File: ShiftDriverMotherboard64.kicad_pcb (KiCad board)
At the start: 2 copper layers, 9 parts, among them U1 ShiftDriver, U2 ShiftDriver, U3 ShiftDriver, U4 ShiftDriver, U5 ShiftDriver, U6 ShiftDriver, U7 ShiftDriver, U8 ShiftDriver, U9 TEENSY_3.6_MINIMAL

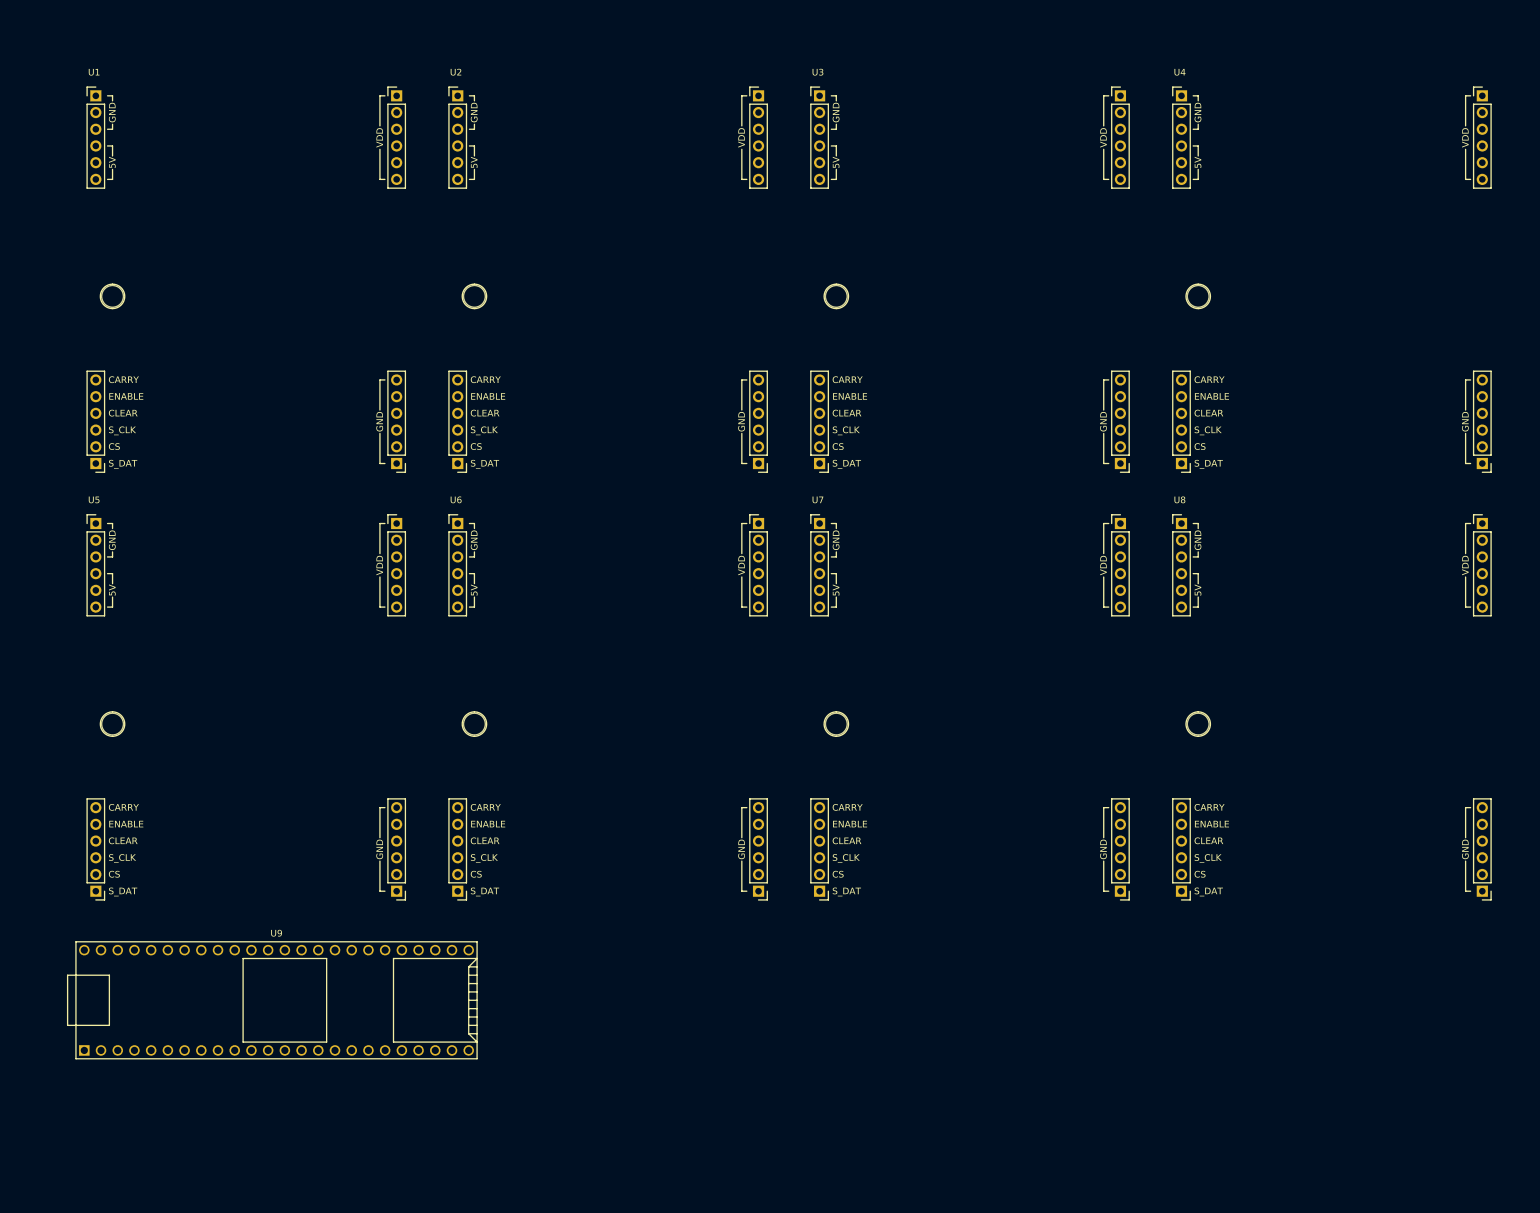
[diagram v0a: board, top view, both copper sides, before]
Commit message: first crack at layout, gonna try laying traces soon
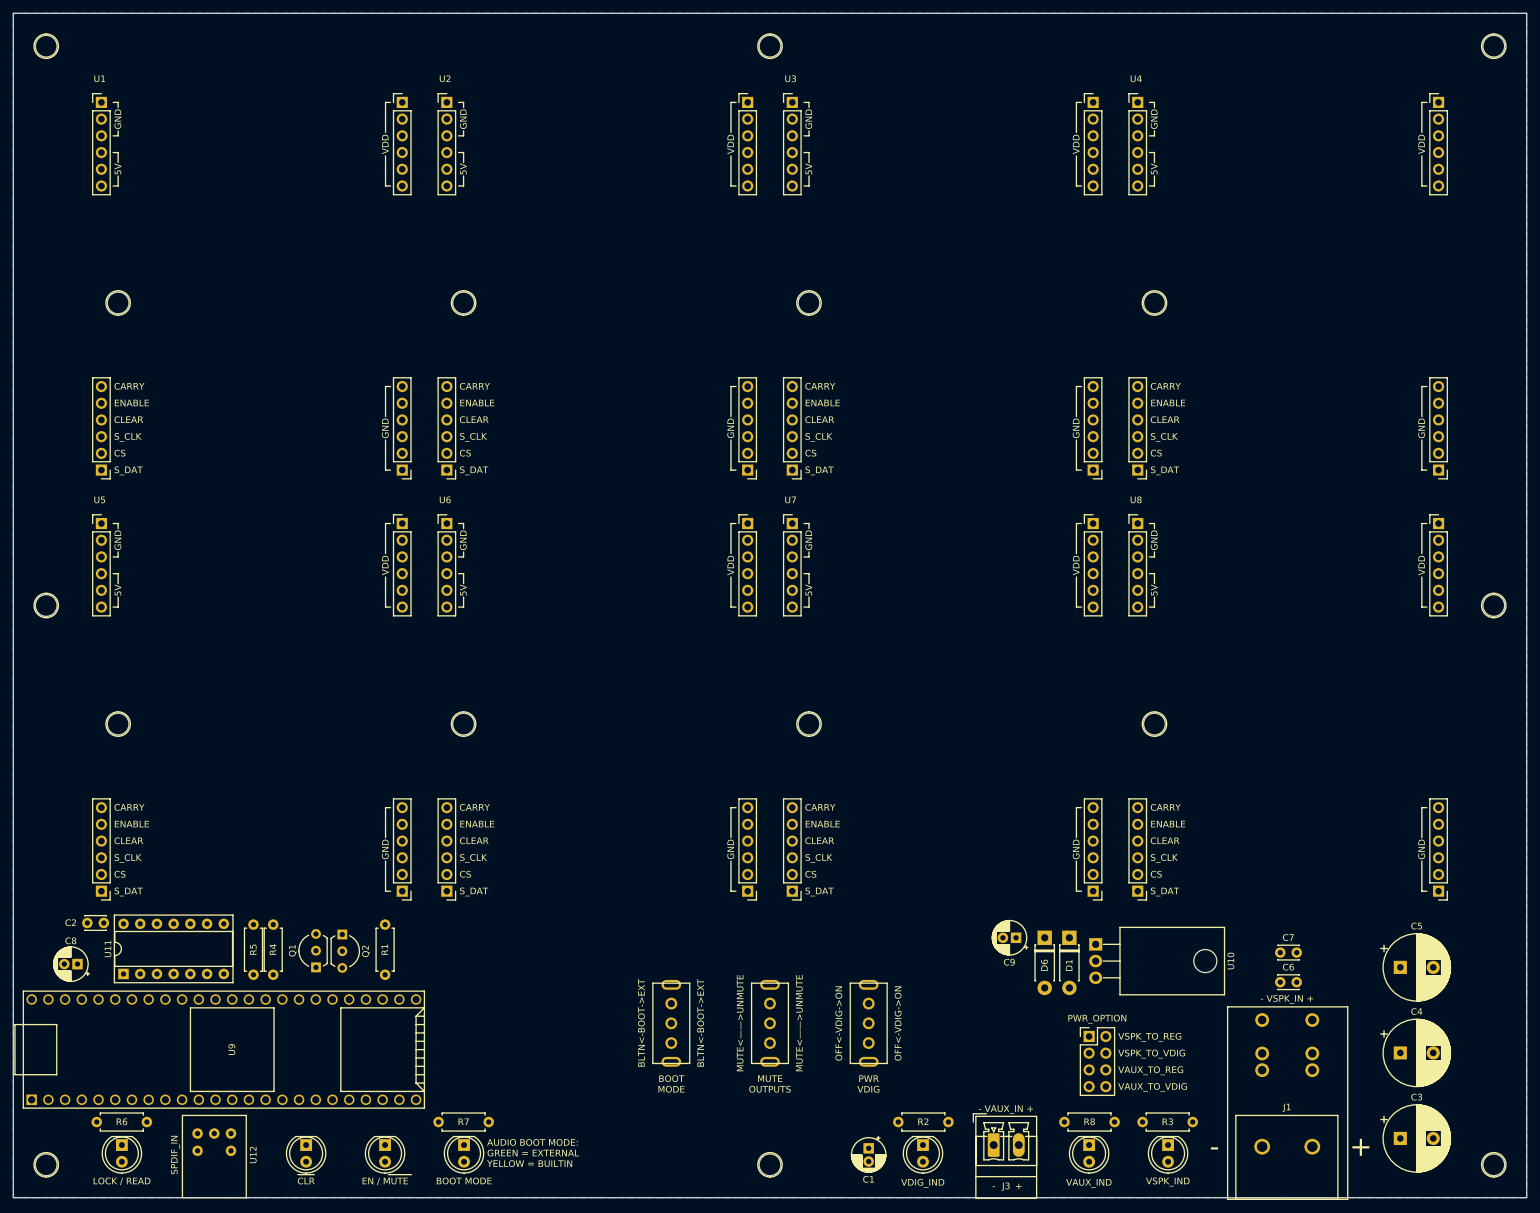
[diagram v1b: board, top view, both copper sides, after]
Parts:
- added C1: 10uf, Capacitor_THT:CP_Radial_D5.0mm_P2.00mm, F.Cu at (140.0, 182.5)
- added C2: 0.1uf, Capacitor_THT:C_Disc_D3.0mm_W2.0mm_P2.50mm, F.Cu at (21.2, 148.2)
- added C3: 470uf, Capacitor_THT:CP_Radial_D10.0mm_P5.00mm, F.Cu at (220.8, 181.0)
- added C4: 470uf, Capacitor_THT:CP_Radial_D10.0mm_P5.00mm, F.Cu at (220.8, 168.0)
- added C5: 470uf, Capacitor_THT:CP_Radial_D10.0mm_P5.00mm, F.Cu at (220.8, 155.0)
- added C6: 0.1uf, Capacitor_THT:C_Disc_D3.0mm_W2.0mm_P2.50mm, F.Cu at (202.6, 157.2)
- added C7: 0.1uf, Capacitor_THT:C_Disc_D3.0mm_W2.0mm_P2.50mm, F.Cu at (202.6, 152.8)
- added C8: 10uf, Capacitor_THT:CP_Radial_D5.0mm_P2.00mm, F.Cu at (19.8, 154.5)
- added C9: 10uf, Capacitor_THT:CP_Radial_D5.0mm_P2.00mm, F.Cu at (162.4, 150.5)
- added D1: 1N4001, Diode_THT:D_DO-41_SOD81_P7.62mm_Horizontal, F.Cu at (170.5, 150.5)
- added D2: TEENSY_PWR_IND, LED_THT:LED_D5.0mm, F.Cu at (148.2, 182.0)
- added D3: VDD_IND, LED_THT:LED_D5.0mm, F.Cu at (185.5, 182.0)
- added D4: CLR_LED, LED_THT:LED_D5.0mm, F.Cu at (54.5, 182.0)
- added D5: EN_LED, LED_THT:LED_D5.0mm, F.Cu at (66.5, 182.0)
- added D6: 1N4001, Diode_THT:D_DO-41_SOD81_P7.62mm_Horizontal, F.Cu at (166.8, 150.5)
- added D7: LOCK_IND, LED_THT:LED_D5.0mm, F.Cu at (26.5, 182.0)
- added D8: BOOT_IND, LED_THT:LED_D5.0mm, F.Cu at (78.5, 182.0)
- added D9: VDIG, LED_THT:LED_D5.0mm, F.Cu at (173.5, 182.0)
- added H3: M3/#4-40, HammerheadAudio:M3_MOUNT, F.Cu at (15.0, 185.0)
- added H3: M3/#4-40, HammerheadAudio:M3_MOUNT, F.Cu at (235.0, 100.0)
- added H3: M3/#4-40, HammerheadAudio:M3_MOUNT, F.Cu at (235.0, 185.0)
- added H3: M3/#4-40, HammerheadAudio:M3_MOUNT, F.Cu at (15.0, 100.0)
- added H3: M3/#4-40, HammerheadAudio:M3_MOUNT, F.Cu at (125.0, 15.0)
- added H3: M3/#4-40, HammerheadAudio:M3_MOUNT, F.Cu at (125.0, 185.0)
- added H3: M3/#4-40, HammerheadAudio:M3_MOUNT, F.Cu at (235.0, 15.0)
- added H3: M3/#4-40, HammerheadAudio:M3_MOUNT, F.Cu at (15.0, 15.0)
- added J1: - VSPK_IN +, HammerheadAudio:ScrewTerm+Phoenix_30A_7.62mm_1x2, F.Cu at (199.8, 163.0)
- added J2: PWR OPTION HEADER, Connector_PinHeader_2.54mm:PinHeader_2x04_P2.54mm_Vertical, F.Cu at (173.5, 165.5)
- added J3: V_TNSY_IN, HammerheadAudio:Phoenix_Stacked, F.Cu at (159.0, 182.0)
- added Q1: Q_NPN_EBC, Package_TO_SOT_THT:TO-92L_Inline_Wide, F.Cu at (56.0, 155.0)
- added Q2: Q_NPN_EBC, Package_TO_SOT_THT:TO-92L_Inline_Wide, F.Cu at (60.0, 150.0)
- added R1: 1k, HammerheadAudio:R_THT_P7.62, F.Cu at (66.5, 148.5)
- added R2: 220, HammerheadAudio:R_THT_P7.62, F.Cu at (144.5, 178.5)
- added R3: 220, HammerheadAudio:R_THT_P7.62, F.Cu at (189.2, 178.5)
- added R4: 1k, HammerheadAudio:R_THT_P7.62, F.Cu at (49.5, 148.5)
- added R5: 10k, HammerheadAudio:R_THT_P7.62, F.Cu at (46.5, 148.5)
- added R6: 1k, HammerheadAudio:R_THT_P7.62, F.Cu at (30.3, 178.5)
- added R7: 1k, HammerheadAudio:R_THT_P7.62, F.Cu at (82.2, 178.5)
- added R8: 220, HammerheadAudio:R_THT_P7.62, F.Cu at (169.8, 178.5)
- added SW1: TEENSY_PWR, HammerheadAudio:Tayda_Slide_SPDT, F.Cu at (140.0, 163.5)
- added SW2: BOOT_MODE, HammerheadAudio:Tayda_Slide_SPDT, F.Cu at (110.0, 163.5)
- added SW3: MUTE_SW, HammerheadAudio:Tayda_Slide_SPDT, F.Cu at (125.0, 163.5)
- added U10: LM7805_TO220, Package_TO_SOT_THT:TO-220-3_Horizontal_TabDown, F.Cu at (174.5, 151.5)
- added U11: CD74HC243, Package_DIP:DIP-14_W7.62mm_Socket, F.Cu at (26.8, 156.0)
- added U12: EAPLRAA4, HammerheadAudio:EAPLRAA4, F.Cu at (38.0, 180.2)
- moved U9 11.0 mm to (42.0, 167.5)
- moved U4 6.72 mm to (178.3, 21.0)
- moved U8 6.65 mm to (178.3, 85.0)
- moved U3 4.27 mm to (125.8, 21.0)
- moved U7 4.15 mm to (125.8, 85.0)
- moved U2 1.93 mm to (73.3, 21.0)
- moved U6 1.65 mm to (73.3, 85.0)
- moved U1 1.31 mm to (20.9, 21.0)
- moved U5 0.85 mm to (20.9, 85.0)
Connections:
- U1 pad 1: Net-(U1-Pad1) -> VDD
- U1 pad 2: Net-(U1-Pad2) -> +5V
- U1 pad 3: Net-(U1-Pad3) -> GND
- U1 pad 4: Net-(U1-Pad4) -> D1
- U1 pad 5: Net-(U1-Pad5) -> CS
- U1 pad 6: Net-(U1-Pad6) -> S_CLK
- U1 pad 7: Net-(U1-Pad7) -> CLR
- U1 pad 8: Net-(U1-Pad8) -> EN
- U1 pad 9: Net-(U1-Pad9) -> D2
- U2 pad 1: Net-(U2-Pad1) -> VDD
- U2 pad 2: Net-(U2-Pad2) -> +5V
- U2 pad 3: Net-(U2-Pad3) -> GND
- U2 pad 4: Net-(U2-Pad4) -> D2
- U2 pad 5: Net-(U2-Pad5) -> CS
- U2 pad 6: Net-(U2-Pad6) -> S_CLK
- U2 pad 7: Net-(U2-Pad7) -> CLR
- U2 pad 8: Net-(U2-Pad8) -> EN
- U2 pad 9: Net-(U2-Pad9) -> D3
- U3 pad 1: Net-(U3-Pad1) -> VDD
- U3 pad 2: Net-(U3-Pad2) -> +5V
- U3 pad 3: Net-(U3-Pad3) -> GND
- U3 pad 4: Net-(U3-Pad4) -> D3
- U3 pad 5: Net-(U3-Pad5) -> CS
- U3 pad 6: Net-(U3-Pad6) -> S_CLK
- U3 pad 7: Net-(U3-Pad7) -> CLR
- U3 pad 8: Net-(U3-Pad8) -> EN
- U3 pad 9: Net-(U3-Pad9) -> D4
- U4 pad 1: Net-(U4-Pad1) -> VDD
- U4 pad 2: Net-(U4-Pad2) -> +5V
- U4 pad 3: Net-(U4-Pad3) -> GND
- U4 pad 4: Net-(U4-Pad4) -> D4
- U4 pad 5: Net-(U4-Pad5) -> CS
- U4 pad 6: Net-(U4-Pad6) -> S_CLK
- U4 pad 7: Net-(U4-Pad7) -> CLR
- U4 pad 8: Net-(U4-Pad8) -> EN
- U4 pad 9: Net-(U4-Pad9) -> D5
- U5 pad 1: Net-(U5-Pad1) -> VDD
- U5 pad 2: Net-(U5-Pad2) -> +5V
- U5 pad 3: Net-(U5-Pad3) -> GND
- U5 pad 4: Net-(U5-Pad4) -> D5
- U5 pad 5: Net-(U5-Pad5) -> CS
- U5 pad 6: Net-(U5-Pad6) -> S_CLK
- U5 pad 7: Net-(U5-Pad7) -> CLR
- U5 pad 8: Net-(U5-Pad8) -> EN
- U5 pad 9: Net-(U5-Pad9) -> D6
- U6 pad 1: Net-(U6-Pad1) -> VDD
- U6 pad 2: Net-(U6-Pad2) -> +5V
- U6 pad 3: Net-(U6-Pad3) -> GND
- U6 pad 4: Net-(U6-Pad4) -> D6
- U6 pad 5: Net-(U6-Pad5) -> CS
- U6 pad 6: Net-(U6-Pad6) -> S_CLK
- U6 pad 7: Net-(U6-Pad7) -> CLR
- U6 pad 8: Net-(U6-Pad8) -> EN
- U6 pad 9: Net-(U6-Pad9) -> D7
- U7 pad 1: Net-(U7-Pad1) -> VDD
- U7 pad 2: Net-(U7-Pad2) -> +5V
- U7 pad 3: Net-(U7-Pad3) -> GND
- U7 pad 4: Net-(U7-Pad4) -> D7
- U7 pad 5: Net-(U7-Pad5) -> CS
- U7 pad 6: Net-(U7-Pad6) -> S_CLK
- U7 pad 7: Net-(U7-Pad7) -> CLR
- U7 pad 8: Net-(U7-Pad8) -> EN
- U7 pad 9: Net-(U7-Pad9) -> D8
- U8 pad 1: Net-(U8-Pad1) -> VDD
- U8 pad 2: Net-(U8-Pad2) -> +5V
- U8 pad 3: Net-(U8-Pad3) -> GND
- U8 pad 4: Net-(U8-Pad4) -> D8
- U8 pad 5: Net-(U8-Pad5) -> CS
- U8 pad 6: Net-(U8-Pad6) -> S_CLK
- U8 pad 7: Net-(U8-Pad7) -> CLR
- U8 pad 8: Net-(U8-Pad8) -> EN
- U9 pad 1: Net-(U9-Pad1) -> GND
- U9 pad 11: Net-(U9-Pad11) -> CLR_PIN
- U9 pad 12: Net-(U9-Pad12) -> CS_PIN
- U9 pad 13: Net-(U9-Pad13) -> DAT_PIN
- U9 pad 15: Net-(U9-Pad15) -> +3V3
- U9 pad 34: Net-(U9-Pad34) -> GND
- U9 pad 35: Net-(U9-Pad35) -> CLK_PIN
- U9 pad 36: Net-(U9-Pad36) -> EN_PIN
- U9 pad 37: Net-(U9-Pad37) -> SPDIF
- U9 pad 46: Net-(U9-Pad46) -> +3V3
- U9 pad 48: Net-(U9-Pad48) -> +5V
- U9 pad 7: Net-(U9-Pad7) -> BOOT_IND2
- U9 pad 8: Net-(U9-Pad8) -> BOOT_IND1
- U9 pad 9: Net-(U9-Pad9) -> LOCK_PIN
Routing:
- added copper zone on B.Cu, net GND
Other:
- board outline added: 230 x 180 mm
- board text added: "+"
- board text added: "-"
- board text added: "- VAUX_IN +"
- board text added: "AUDIO BOOT MODE: GREEN = EXTERNAL YELLOW = BUILTIN"
- board text added: "BLTN<-BOOT->EXT"
- board text added: "BOOT MODE"
- board text added: "CLR"
- board text added: "EN / MUTE"
- board text added: "LOCK / READ"
- board text added: "MUTE OUTPUTS"
- board text added: "MUTE<——>UNMUTE"
- board text added: "OFF<-VDIG->ON"
- board text added: "PWR VDIG"
- board text added: "PWR_OPTION"
- board text added: "SPDIF_IN"
- board text added: "VAUX_IND"
- board text added: "VAUX_TO_REG"
- board text added: "VAUX_TO_VDIG"
- board text added: "VDIG_IND"
- board text added: "VSPK_IND"
- board text added: "VSPK_TO_REG"
- board text added: "VSPK_TO_VDIG"
